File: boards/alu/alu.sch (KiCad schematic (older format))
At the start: 80 parts, among them U1 28C256, U2 74ACT08, U3 28C256, U4 74ACT00, U5 74ACT02

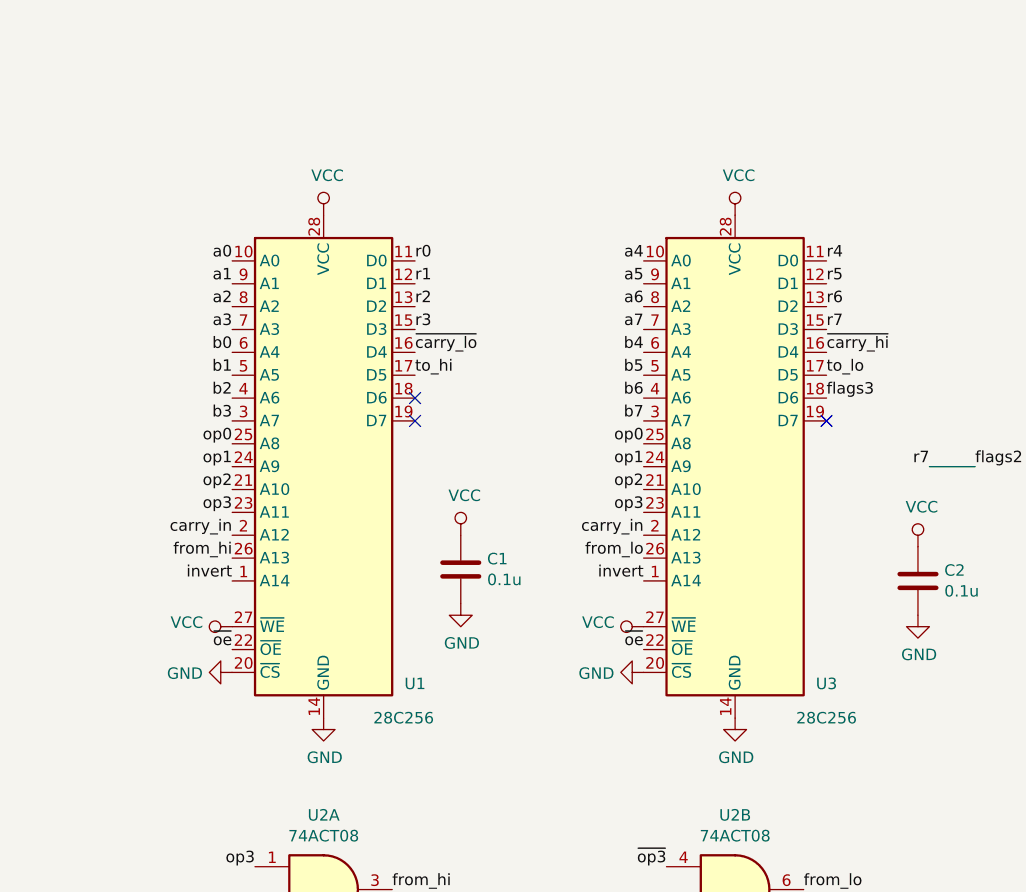
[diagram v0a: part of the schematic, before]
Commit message: PLCC-32 socket footprint
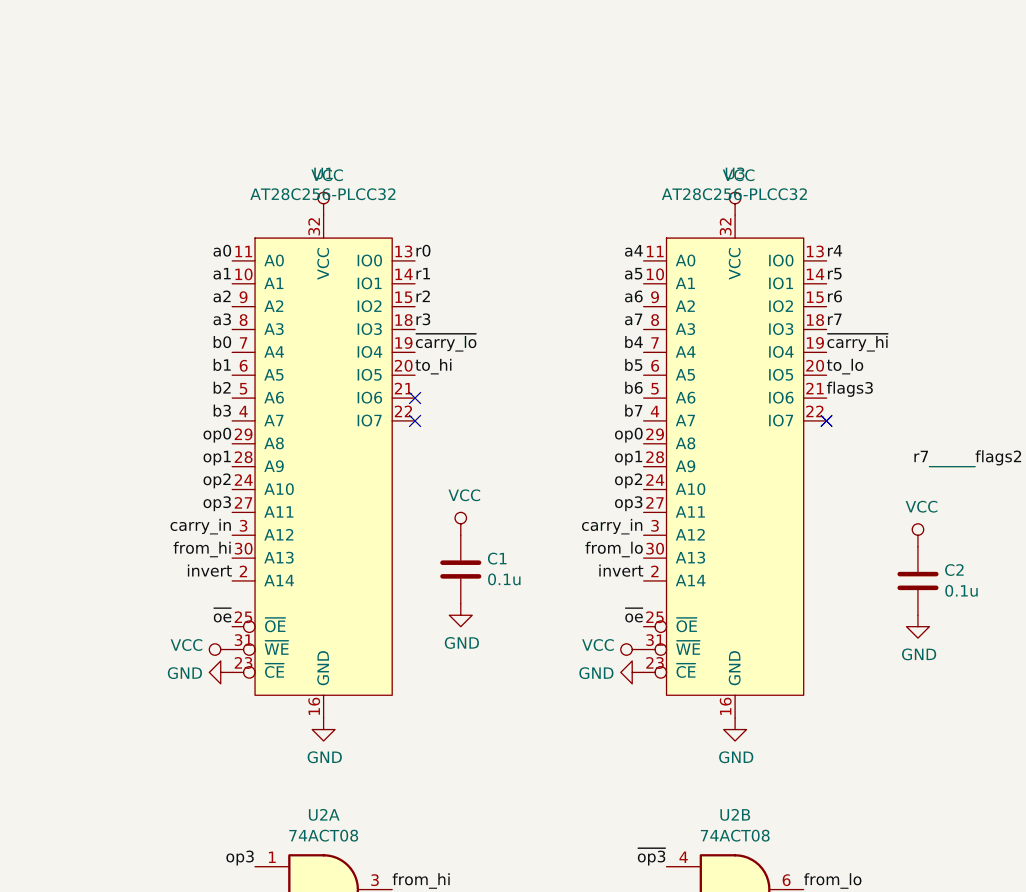
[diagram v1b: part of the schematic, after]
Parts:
- removed U1, U3: 28C256, Package_LCC:PLCC-28_SMD-Socket, symbol Memory_EEPROM:28C256
- added U1, U3: AT28C256-PLCC32, missing:PLCC-32_SMD_Socket, symbol missing:AT28C256-PLCC32
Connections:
- net GND: now also U1.16 (GND), U1.23 (~CE), U3.16 (GND), U3.23 (~CE)
- net VCC: now also U1.31 (~WE), U1.32 (VCC), U3.31 (~WE), U3.32 (VCC)
- net a0: now also U1.11 (A0)
- net a1: now also U1.10 (A1)
- net a2: now also U1.9 (A2)
- net a3: now also U1.8 (A3)
- net a4: now also U3.11 (A0)
- net a5: now also U3.10 (A1)
- net a6: now also U3.9 (A2)
- net a7: now also U3.8 (A3)
- net b0: now also U1.7 (A4)
- net b1: now also U1.6 (A5)
- net b2: now also U1.5 (A6)
- net b3: now also U1.4 (A7)
- net b4: now also U3.7 (A4)
- net b5: now also U3.6 (A5)
- net b6: now also U3.5 (A6)
- net b7: now also U3.4 (A7)
- net carry_in: now also U1.3 (A12), U3.3 (A12)
- net flags2: now also U3.18 (IO3)
- net flags3: now also U3.21 (IO6)
- net from_hi: now also U1.30 (A13)
- net from_lo: now also U3.30 (A13)
- net invert: now also U1.2 (A14), U3.2 (A14)
- net op0: now also U1.29 (A8), U3.29 (A8)
- net op1: now also U1.28 (A9), U3.28 (A9)
- net op2: now also U1.24 (A10), U3.24 (A10)
- net op3: now also U1.27 (A11), U3.27 (A11)
- net r0: now also U1.13 (IO0)
- net r1: now also U1.14 (IO1)
- net r2: now also U1.15 (IO2)
- net r3: now also U1.18 (IO3)
- net r4: now also U3.13 (IO0)
- net r5: now also U3.14 (IO1)
- net r6: now also U3.15 (IO2)
- net to_hi: now also U1.20 (IO5)
- net to_lo: now also U3.20 (IO5)
- net ~carry_hi: now also U3.19 (IO4)
- net ~carry_lo: now also U1.19 (IO4)
- net ~oe: now also U1.25 (~OE), U3.25 (~OE)
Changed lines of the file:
@@
 Comment4 ""
 $EndDescr
-$Comp
-L Memory_EEPROM:28C256 U1
-U 1 1 5FC22E82
-P 6500 3650
-F 0 "U1" H 6900 2700 50  0000 C CNN
-F 1 "28C256" H 6850 2550 50  0000 C CNN
-F 2 "Package_LCC:PLCC-28_SMD-Socket" H 6500 3650 50  0001 C CNN
-F 3 "http://ww1.microchip.com/downloads/en/DeviceDoc/doc0006.pdf" H 6500 3650 50  0001 C CNN
-	1    6500 3650
-	1    0    0    -1
-$EndComp
 Text Label 6100 2750 2    50   ~ 0
 a0
@@
 Text Label 8700 3250 0    50   ~ 0
 to_lo
-$Comp
-L Memory_EEPROM:28C256 U3
-U 1 1 5FC23A8E
-P 8300 3650
-F 0 "U3" H 8700 2700 50  0000 C CNN
-F 1 "28C256" H 8700 2550 50  0000 C CNN
-F 2 "Package_LCC:PLCC-28_SMD-Socket" H 8300 3650 50  0001 C CNN
-F 3 "http://ww1.microchip.com/downloads/en/DeviceDoc/doc0006.pdf" H 8300 3650 50  0001 C CNN
-	1    8300 3650
-	1    0    0    -1
-$EndComp
 NoConn ~ 8700 3450
 $Comp
@@
 L power:VCC #PWR01
 U 1 1 5FC2D9E5
-P 6100 4350
-F 0 "#PWR01" H 6100 4200 50  0001 C CNN
-F 1 "VCC" V 6118 4477 50  0000 L CNN
-F 2 "" H 6100 4350 50  0001 C CNN
-F 3 "" H 6100 4350 50  0001 C CNN
-	1    6100 4350
+P 6100 4450
+F 0 "#PWR01" H 6100 4300 50  0001 C CNN
+F 1 "VCC" V 6118 4577 50  0000 L CNN
+F 2 "" H 6100 4450 50  0001 C CNN
+F 3 "" H 6100 4450 50  0001 C CNN
+	1    6100 4450
 	0    -1   -1   0
 $EndComp
@@
 L power:VCC #PWR07
 U 1 1 5FC2E2AC
-P 7900 4350
-F 0 "#PWR07" H 7900 4200 50  0001 C CNN
-F 1 "VCC" V 7918 4477 50  0000 L CNN
-F 2 "" H 7900 4350 50  0001 C CNN
-F 3 "" H 7900 4350 50  0001 C CNN
-	1    7900 4350
+P 7900 4450
+F 0 "#PWR07" H 7900 4300 50  0001 C CNN
+F 1 "VCC" V 7918 4577 50  0000 L CNN
+F 2 "" H 7900 4450 50  0001 C CNN
+F 3 "" H 7900 4450 50  0001 C CNN
+	1    7900 4450
 	0    -1   -1   0
 $EndComp
@@
 Text Label 12950 3100 0    50   ~ 0
 flags[0..3]
-Text Label 7900 4450 2    50   ~ 0
+Text Label 7900 4350 2    50   ~ 0
 ~oe
-Text Label 6100 4450 2    50   ~ 0
+Text Label 6100 4350 2    50   ~ 0
 ~oe
 Text Label 9350 3650 0    50   ~ 0
@@
 Wire Bus Line
 	10750 1700 10750 3100
+$Comp
+L missing:AT28C256-PLCC32 U1
+U 1 1 60197966
+P 6500 3650
+F 0 "U1" H 6500 4931 50  0000 C CNN
+F 1 "AT28C256-PLCC32" H 6500 4840 50  0000 C CNN
+F 2 "missing:PLCC-32_SMD_Socket" H 6750 4000 50  0001 C CNN
+F 3 "http://ww1.microchip.com/downloads/en/DeviceDoc/doc0006.pdf" H 6750 4000 50  0001 C CNN
+	1    6500 3650
+	1    0    0    -1
+$EndComp
+$Comp
+L missing:AT28C256-PLCC32 U3
+U 1 1 60199147
+P 8300 3650
+F 0 "U3" H 8300 4931 50  0000 C CNN
+F 1 "AT28C256-PLCC32" H 8300 4840 50  0000 C CNN
+F 2 "missing:PLCC-32_SMD_Socket" H 8550 4000 50  0001 C CNN
+F 3 "http://ww1.microchip.com/downloads/en/DeviceDoc/doc0006.pdf" H 8550 4000 50  0001 C CNN
+	1    8300 3650
+	1    0    0    -1
+$EndComp
 $EndSCHEMATC
